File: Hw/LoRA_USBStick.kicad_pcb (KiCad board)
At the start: 2 copper layers, 61.5 x 18.7 mm, 17 parts, among them J10 USB_B, J4 SWD, SW1 RST, U1 ATSAMD21E, U2 RFM95W-868S2, U7 AP2114H-3.3TRG1

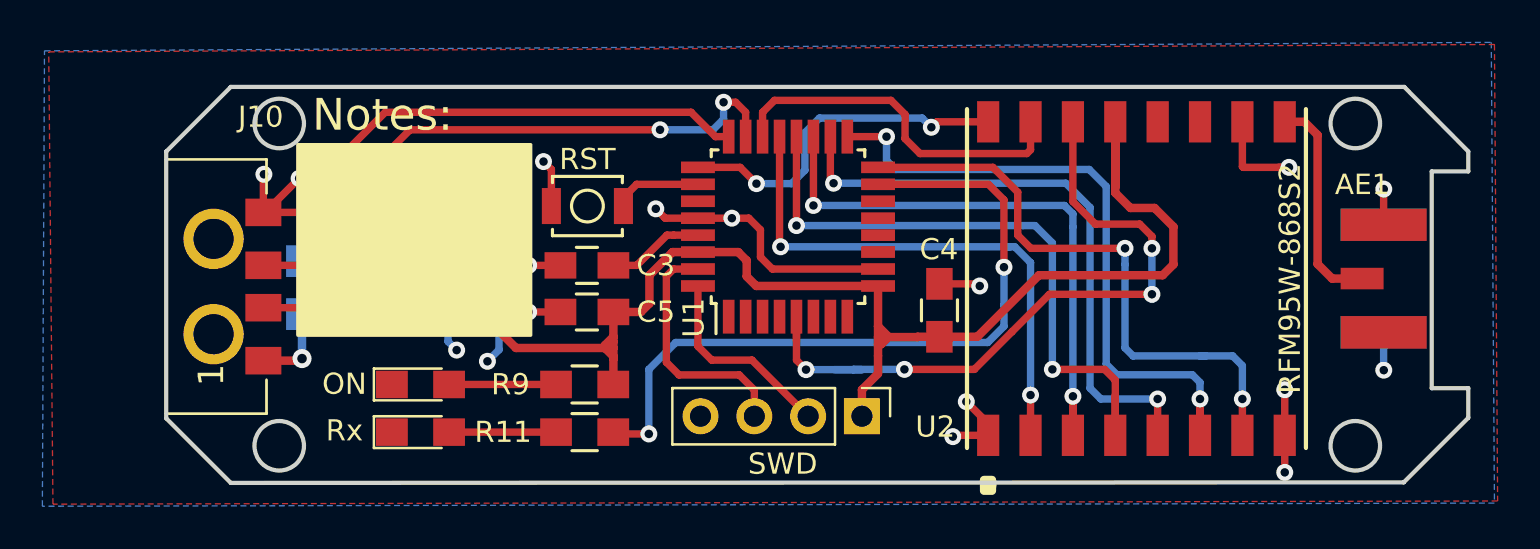
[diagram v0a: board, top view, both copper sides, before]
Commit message: Update V3.0
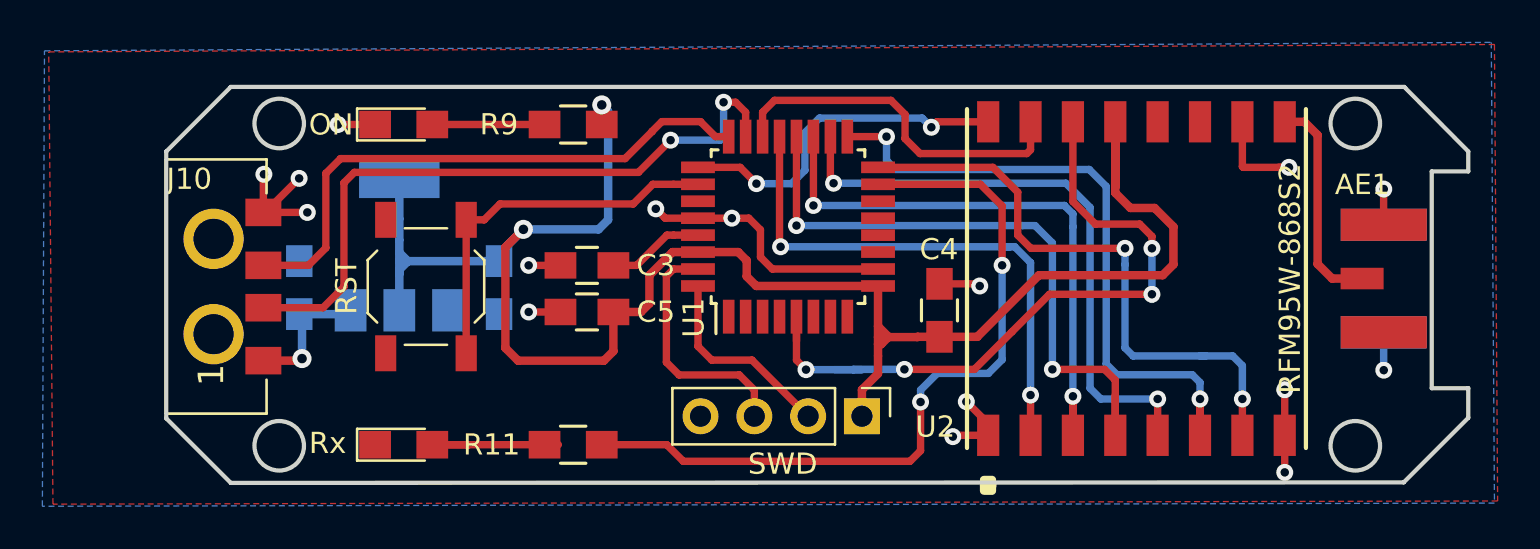
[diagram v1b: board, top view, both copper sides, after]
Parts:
- SW1: footprint Buttons_Switches_SMD:SW_SPST_B3U-1000P -> Button_Switch_SMD:SW_SPST_TL3342
- moved D6 12.3 mm to (128.0, 106.5)
- moved R9 12.3 mm to (136.0, 106.5)
- moved SW1 8.52 mm to (129.1, 114.2), turned to 270 degrees
- moved D7 0.99 mm to (128.0, 121.7)
- moved R11 0.80 mm to (136.0, 121.7)
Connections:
- net /DI1 renamed Net-(U1-Pad3)
- net /DI2 renamed Net-(U1-Pad2)
- net /DI3 renamed Net-(U1-Pad1)
- net /DO1 renamed Net-(U1-Pad8)
- net /DO2 renamed Net-(U1-Pad7)
- net /DO3 renamed Net-(U1-Pad6)
- net /Rx renamed Net-(U1-Pad14)
- net /Tx renamed Net-(U1-Pad13)
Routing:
- net /RST: track 4.18 -> 17.9 mm
- net GND: track 46.7 -> 42.0 mm, vias 18 -> 16
- net Net-(D7-Pad2): track 5.05 -> 6.90 mm
- net /Rx_LED: track 34.6 -> 36.4 mm
- net /D+: track 28.2 -> 27.1 mm
- net +3V3: track 88.8 -> 88.7 mm, vias 3 -> 2
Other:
- board text removed: "Notes:"
